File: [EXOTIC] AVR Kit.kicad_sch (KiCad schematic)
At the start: 21 parts, among them J2 AVR-ISP-10, J3 USB_B, J4 Conn_01x08_Socket, J5 Conn_01x08_Socket, J6 Conn_01x09_Socket, J7 Conn_01x07_Socket, J8 ICSP_Connector, SW1 SW_Push, U1 ATmega32A-P, U6 CH340C, Y1 16 MHz

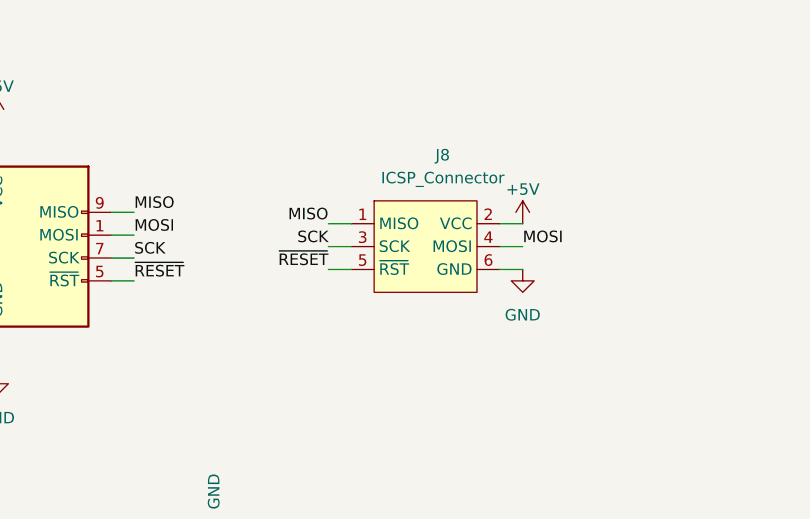
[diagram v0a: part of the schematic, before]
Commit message: Rev. 3
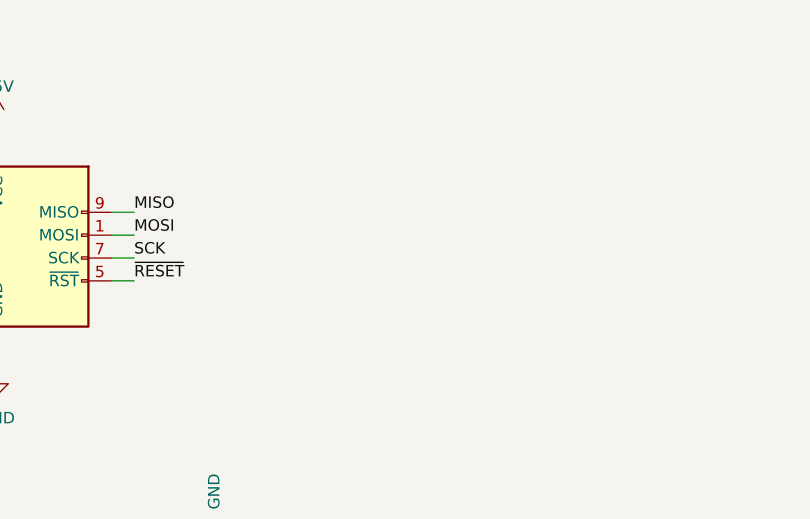
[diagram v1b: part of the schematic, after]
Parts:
- removed J8: ICSP_Connector, Connector_PinHeader_2.54mm:PinHeader_2x03_P2.54mm_Vertical, symbol PCM_SL_Connectors:ICSP_Connector
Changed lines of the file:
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@@
-    (stroke (width 0) (type default))
-  )
-  (wire (pts (xy 189.23 52.07) (xy 191.77 52.07))
     (stroke (width 0) (type default))
   )
@@
     (stroke (width 0) (type default))
   )
-  (wire (pts (xy 210.82 46.99) (xy 208.28 46.99))
-    (stroke (width 0) (type default))
-  )
   (wire (pts (xy 91.44 111.76) (xy 105.41 111.76))
     (stroke (width 0) (type default))
@@
     (stroke (width 0) (type default))
   )
-  (wire (pts (xy 210.82 52.07) (xy 208.28 52.07))
-    (stroke (width 0) (type default))
-  )
   (wire (pts (xy 76.2 147.32) (xy 76.2 148.59))
     (stroke (width 0) (type default))
@@
     (stroke (width 0) (type default))
   )
-  (wire (pts (xy 189.23 46.99) (xy 191.77 46.99))
-    (stroke (width 0) (type default))
-  )
   (wire (pts (xy 58.42 44.45) (xy 60.96 44.45))
     (stroke (width 0) (type default))
@@
     (stroke (width 0) (type default))
   )
-  (wire (pts (xy 189.23 49.53) (xy 191.77 49.53))
-    (stroke (width 0) (type default))
-  )
   (wire (pts (xy 154.94 115.57) (xy 157.48 115.57))
     (stroke (width 0) (type default))
@@
   )
   (wire (pts (xy 91.44 101.6) (xy 105.41 101.6))
-    (stroke (width 0) (type default))
-  )
-  (wire (pts (xy 210.82 49.53) (xy 208.28 49.53))
     (stroke (width 0) (type default))
   )
@@
     (effects (font (size 1.27 1.27)) (justify left bottom))
   )
-  (label "MOSI" (at 210.82 49.53 0) (fields_autoplaced)
-    (effects (font (size 1.27 1.27)) (justify left bottom))
-  )
   (label "PD7" (at 101.6 96.52 0) (fields_autoplaced)
     (effects (font (size 1.27 1.27)) (justify left bottom))
@@
     (effects (font (size 1.27 1.27)) (justify left bottom))
   )
-  (label "SCK" (at 189.23 49.53 180) (fields_autoplaced)
-    (effects (font (size 1.27 1.27)) (justify right bottom))
-  )
   (label "PA3" (at 93.98 60.96 0) (fields_autoplaced)
     (effects (font (size 1.27 1.27)) (justify left bottom))
@@
   (label "PA4" (at 93.98 63.5 0) (fields_autoplaced)
     (effects (font (size 1.27 1.27)) (justify left bottom))
-  )
-  (label "MISO" (at 189.23 46.99 180) (fields_autoplaced)
-    (effects (font (size 1.27 1.27)) (justify right bottom))
   )
   (label "TDO" (at 93.98 109.22 0) (fields_autoplaced)
@@
   (label "PB1" (at 93.98 78.74 0) (fields_autoplaced)
     (effects (font (size 1.27 1.27)) (justify left bottom))
-  )
-  (label "~{RESET}" (at 189.23 52.07 180) (fields_autoplaced)
-    (effects (font (size 1.27 1.27)) (justify right bottom))
   )
   (label "~{RESET}" (at 55.88 53.34 180) (fields_autoplaced)
@@
     )
   )
-  (symbol (lib_id "PCM_SL_Connectors:ICSP_Connector") (at 199.39 49.53 0) (unit 1)
-    (in_bom yes) (on_board yes) (dnp no) (fields_autoplaced)
-    (property "Reference" "J8" (at 201.93 39.37 0)
-      (effects (font (size 1.27 1.27)))
-    )
-    (property "Value" "ICSP_Connector" (at 201.93 41.91 0)
-      (effects (font (size 1.27 1.27)))
-    )
-    (property "Footprint" "Connector_PinHeader_2.54mm:PinHeader_2x03_P2.54mm_Vertical" (at 195.58 46.99 0)
-      (effects (font (size 1.27 1.27)) hide)
-    )
-    (property "Datasheet" "" (at 195.58 46.99 0)
-      (effects (font (size 1.27 1.27)) hide)
-    )
-    (pin "3")
-    (pin "6")
-    (pin "5")
-    (pin "1")
-    (pin "4")
-    (pin "2")
-    (instances
-      (project "[EXOTIC] AVR Kit"
-        (path "/bd689b4b-40d7-46ba-91b6-965ce30f8212"
-          (reference "J8") (unit 1)
-        )
-      )
-    )
-  )
   (symbol (lib_id "Device:R") (at 60.96 35.56 0) (unit 1)
     (in_bom yes) (on_board yes) (dnp no) (fields_autoplaced)
@@
     )
   )
-  (symbol (lib_id "power:GND") (at 210.82 52.07 0) (unit 1)
-    (in_bom yes) (on_board yes) (dnp no) (fields_autoplaced)
-    (property "Reference" "#PWR033" (at 210.82 58.42 0)
-      (effects (font (size 1.27 1.27)) hide)
-    )
-    (property "Value" "GND" (at 210.82 57.15 0)
-      (effects (font (size 1.27 1.27)))
-    )
-    (property "Footprint" "" (at 210.82 52.07 0)
-      (effects (font (size 1.27 1.27)) hide)
-    )
-    (property "Datasheet" "" (at 210.82 52.07 0)
-      (effects (font (size 1.27 1.27)) hide)
-    )
-    (pin "1")
-    (instances
-      (project "[EXOTIC] AVR Kit"
-        (path "/bd689b4b-40d7-46ba-91b6-965ce30f8212"
-          (reference "#PWR033") (unit 1)
-        )
-      )
-      (project "ATMEGA32A Development Board"
-        (path "/e232854a-3fe0-4443-9abe-081b69d86c79"
-          (reference "#PWR018") (unit 1)
-        )
-      )
-    )
-  )
   (symbol (lib_id "Connector:USB_B") (at 199.39 102.87 0) (mirror y) (unit 1)
     (in_bom yes) (on_board yes) (dnp no)
@@
         )
       )
-    )
-  )
-  (symbol (lib_id "power:+5V") (at 210.82 46.99 0) (unit 1)
-    (in_bom yes) (on_board yes) (dnp no) (fields_autoplaced)
-    (property "Reference" "#PWR032" (at 210.82 50.8 0)
-      (effects (font (size 1.27 1.27)) hide)
-    )
-    (property "Value" "+5V" (at 210.82 43.18 0)
-      (effects (font (size 1.27 1.27)))
-    )
-    (property "Footprint" "" (at 210.82 46.99 0)
-      (effects (font (size 1.27 1.27)) hide)
-    )
-    (property "Datasheet" "" (at 210.82 46.99 0)
-      (effects (font (size 1.27 1.27)) hide)
-    )
-    (pin "1")
-    (instances
-      (project "[EXOTIC] AVR Kit"
-        (path "/bd689b4b-40d7-46ba-91b6-965ce30f8212"
-          (reference "#PWR032") (unit 1)
-        )
-      )
-      (project "ATMEGA32A Development Board"
-        (path "/e232854a-3fe0-4443-9abe-081b69d86c79"
-          (reference "#PWR012") (unit 1)
-        )
-      )

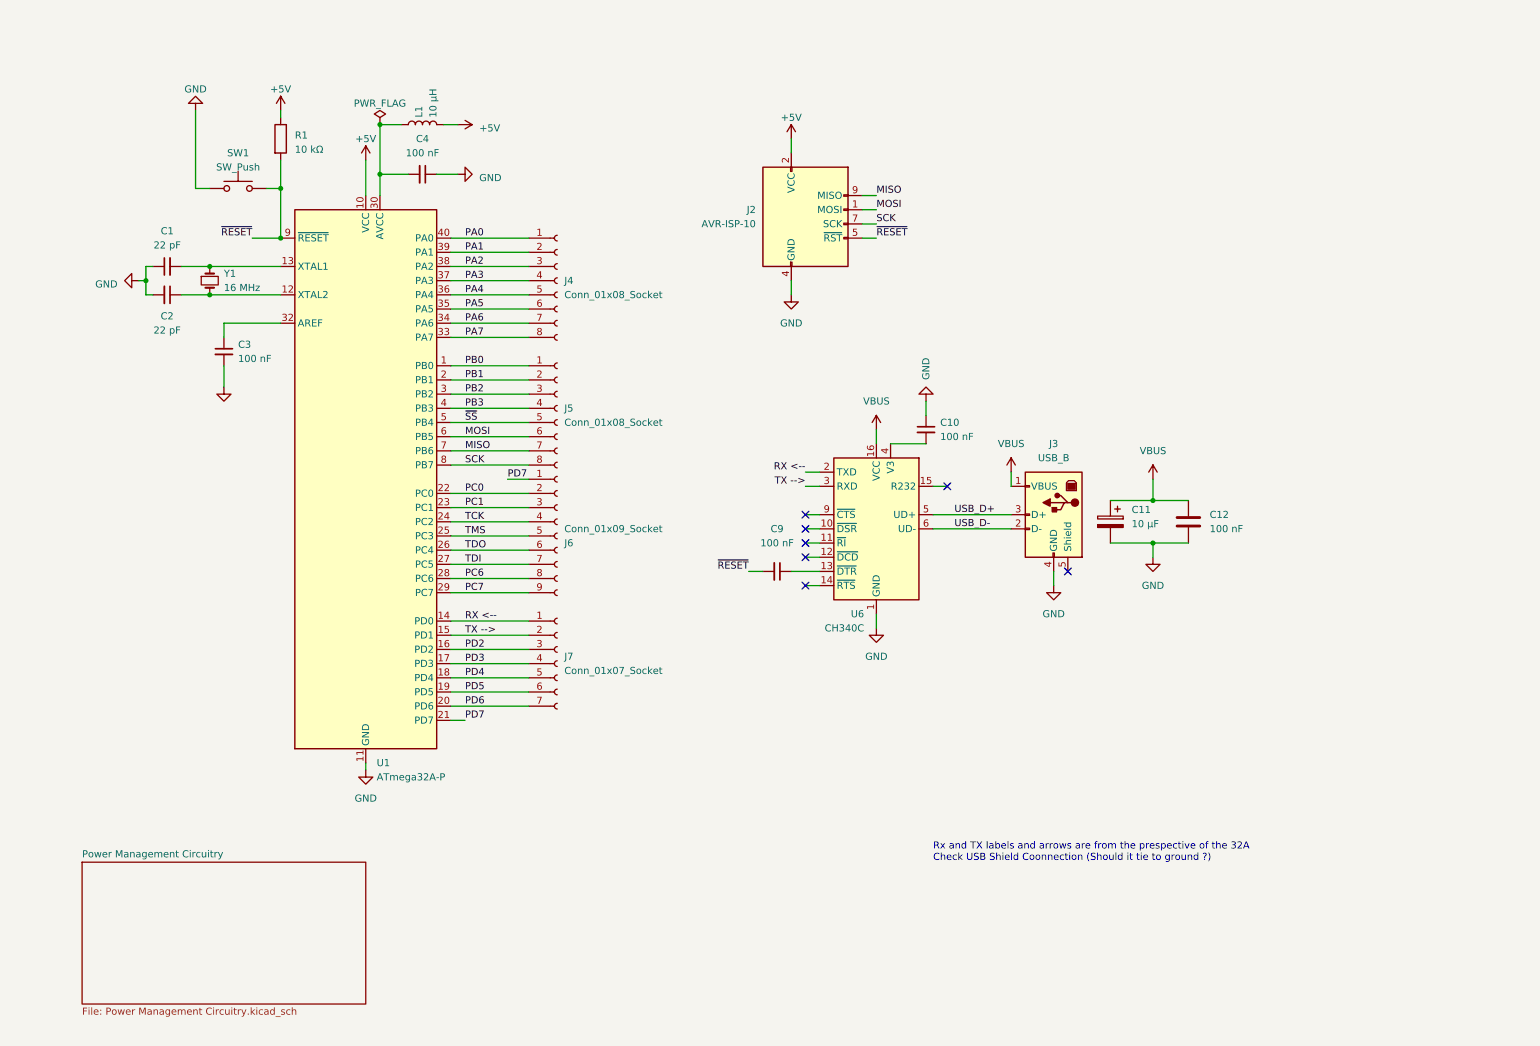
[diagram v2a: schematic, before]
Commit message: Rev 3.2
Cleaned Up Schematic
Revised Layout
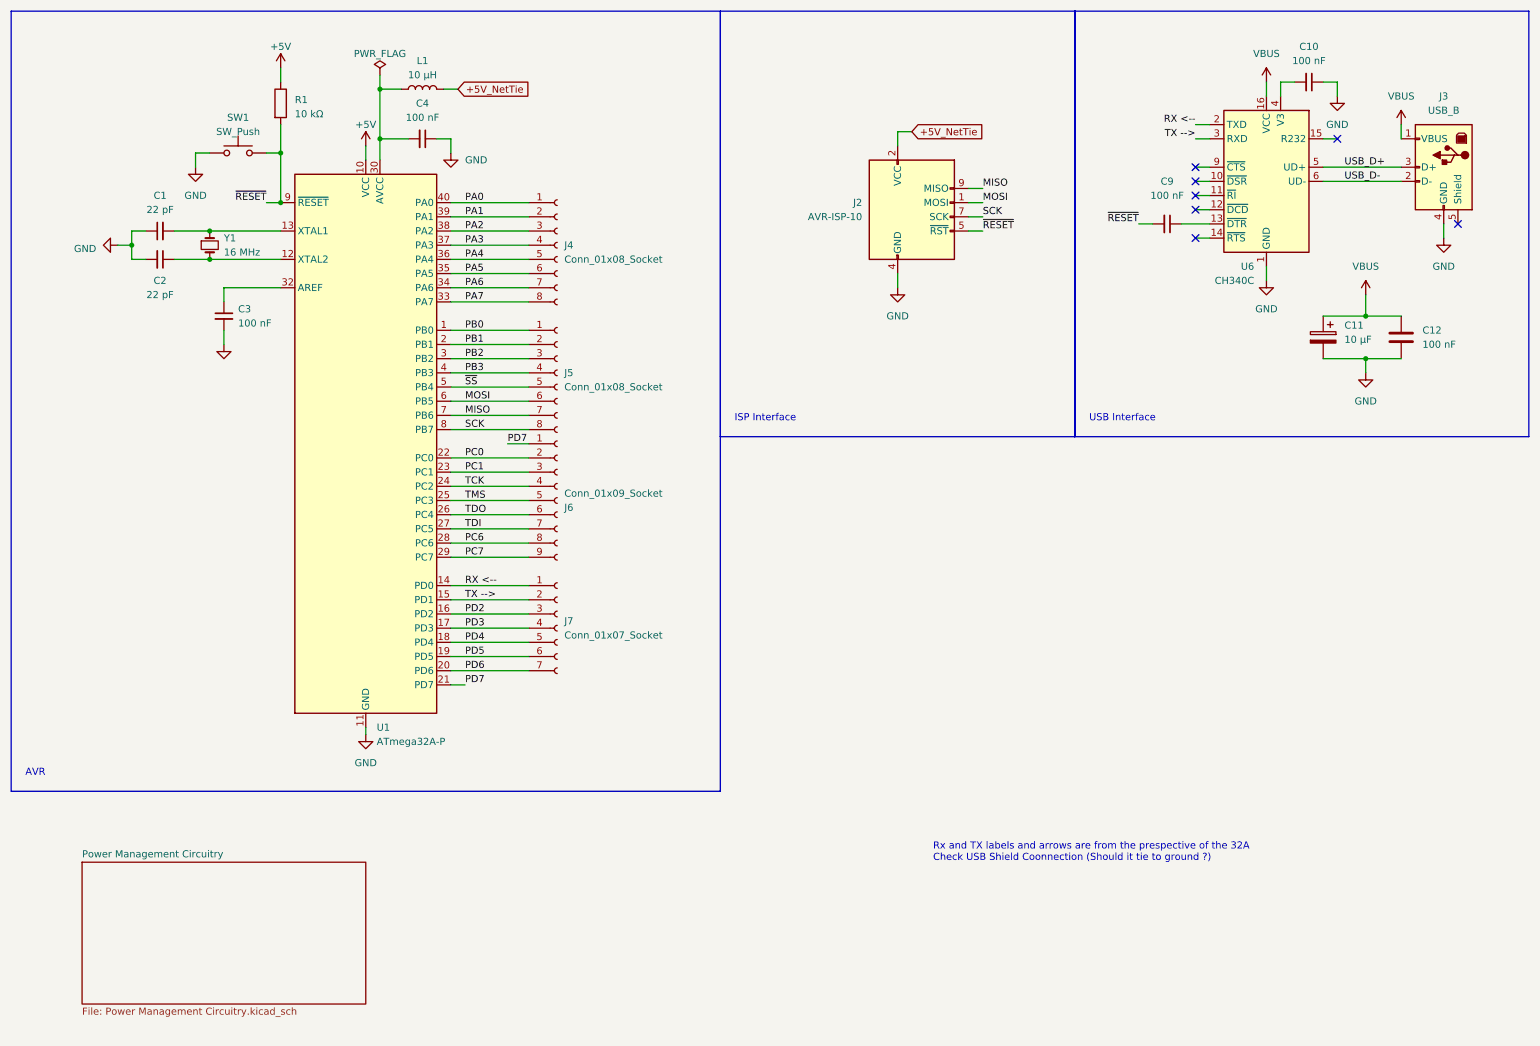
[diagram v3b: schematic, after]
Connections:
- net +5V: no longer J2.2 (VCC), L1.2
- new net +5V_NetTie: J2.2 (VCC), L1.2
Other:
- note added: "AVR"
- note added: "ISP Interface"
- note added: "USB Interface"
- moved on the sheet: C1, C10, C11, C12, C2, C3, C4, C9, J2, J3, J4, J5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

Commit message: Schematic Organization
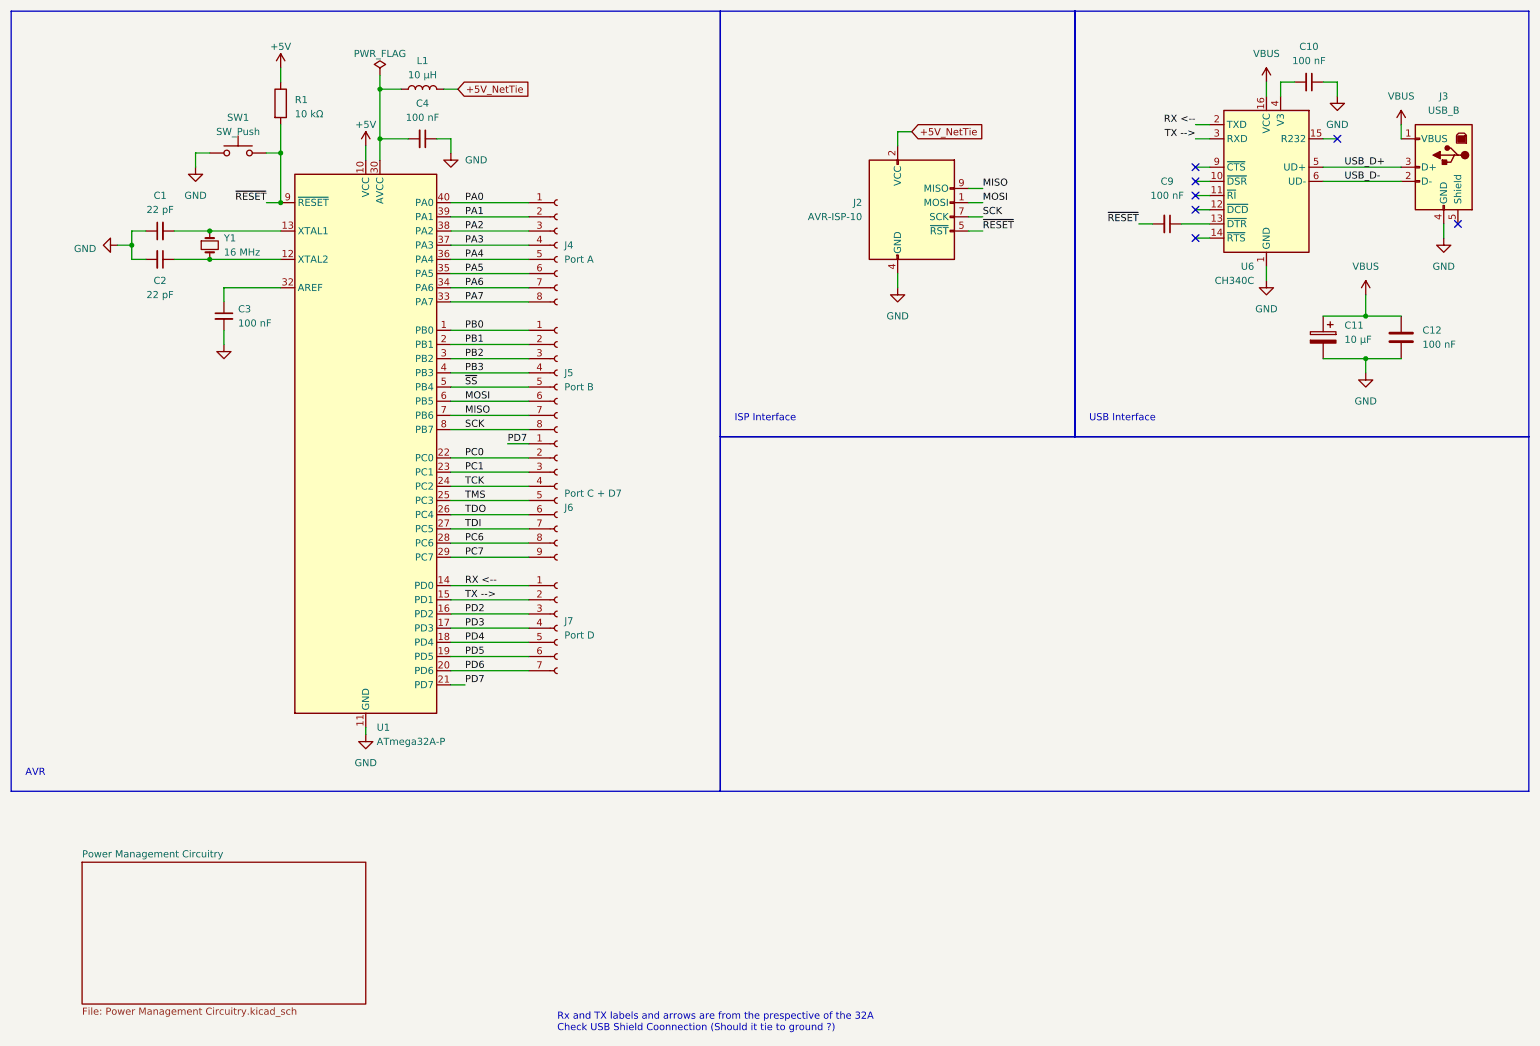
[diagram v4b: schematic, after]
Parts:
- J4: value Conn_01x08_Socket -> Port A
- J5: value Conn_01x08_Socket -> Port B
- J6: value Conn_01x09_Socket -> Port C + D7
- J7: value Conn_01x07_Socket -> Port D
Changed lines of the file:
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@@
+    (fill (type none))
+  )
+  (rectangle (start 139.7 88.9) (end 284.48 152.4)
+    (stroke (width 0) (type default))
     (fill (type none))
   )
@@
   )
   (text "Rx and TX labels and arrows are from the prespective of the 32A\nCheck USB Shield Coonnection (Should it tie to ground ?)"
-    (at 177.8 165.1 0)
+    (at 110.49 195.58 0)
     (effects (font (size 1.27 1.27)) (justify left bottom))
   )
@@
       (effects (font (size 1.27 1.27)) (justify left))
     )
-    (property "Value" "Conn_01x08_Socket" (at 111.76 80.01 0)
+    (property "Value" "Port B" (at 111.76 80.01 0)
       (effects (font (size 1.27 1.27)) (justify left))
     )
@@
       (effects (font (size 1.27 1.27)) (justify left))
     )
-    (property "Value" "Conn_01x09_Socket" (at 111.76 99.06 0)
+    (property "Value" "Port C + D7" (at 111.76 99.06 0)
       (effects (font (size 1.27 1.27)) (justify left))
     )
@@
       (effects (font (size 1.27 1.27)) (justify left))
     )
-    (property "Value" "Conn_01x08_Socket" (at 111.76 57.15 0)
+    (property "Value" "Port A" (at 111.76 57.15 0)
       (effects (font (size 1.27 1.27)) (justify left))
     )
@@
       (effects (font (size 1.27 1.27)) (justify left))
     )
-    (property "Value" "Conn_01x07_Socket" (at 111.76 124.46 0)
-      (effects (font (size 1.27 1.27)) (justify left))
-    )
+    (property "Value" "Port D" (at 111.76 124.46 0)
+      (effects (font (size 1.27 1.27)) (justify left))
+    )
